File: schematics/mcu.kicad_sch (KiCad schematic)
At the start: 7 parts, among them SW1 SW_Push, U2 STM32F103C8Tx, Y1 ECS-2520MV-xxx-xx

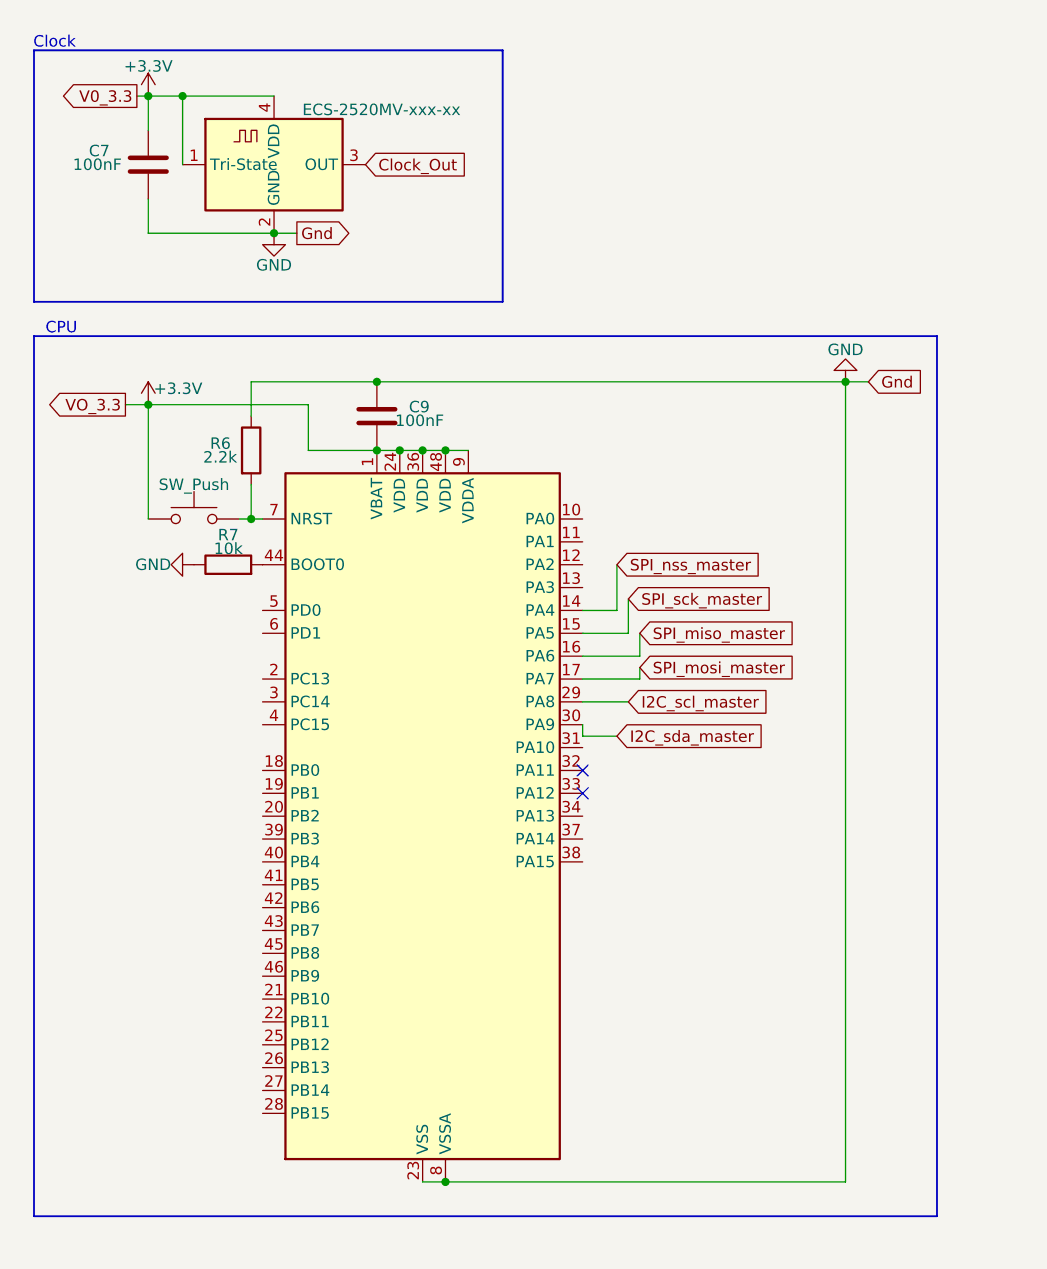
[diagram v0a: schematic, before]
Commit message: 2026-02-25 | Mi
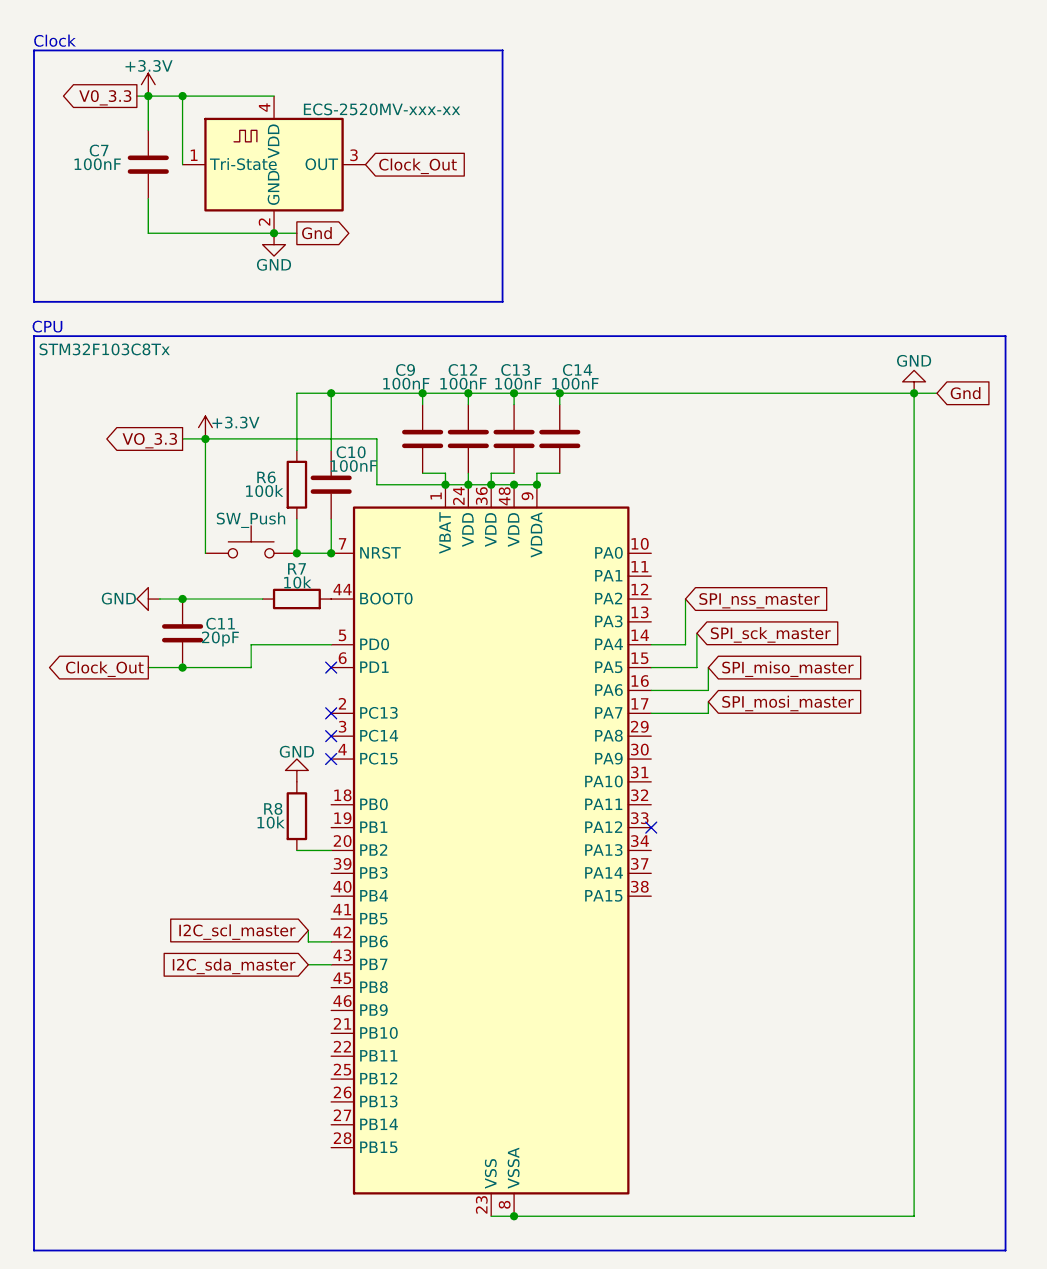
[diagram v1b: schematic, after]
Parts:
- added C10, C12, C13, C14: 100nF, Capacitor_SMD:C_0805_2012Metric, symbol Device:C
- added C11: 20pF, Capacitor_SMD:C_0805_2012Metric, symbol Device:C
- added R8: 10k, Resistor_SMD:R_0402_1005Metric, symbol Device:R
- R6: value 2.2k -> 100k
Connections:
- net +3.3V: now also C12.2, C13.2, C14.2
- net Clock_Out: now also U2.5 (PD0), C11.2
- net GND: now also C10.1, C11.1, C12.1, C13.1, C14.1, R8.1
- net I2C_scl_master: now also U2.42 (PB6); no longer U2.29 (PA8)
- net I2C_sda_master: now also U2.43 (PB7); no longer U2.30 (PA9)
- net at R6.2, SW1.2, U2.7 (NRST): now also C10.2
- net at U2.20 (PB2): now also R8.2
- no-connect marks 2 -> 5
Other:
- moved on the sheet: R6, R7

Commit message: 2026-02-26 | Do
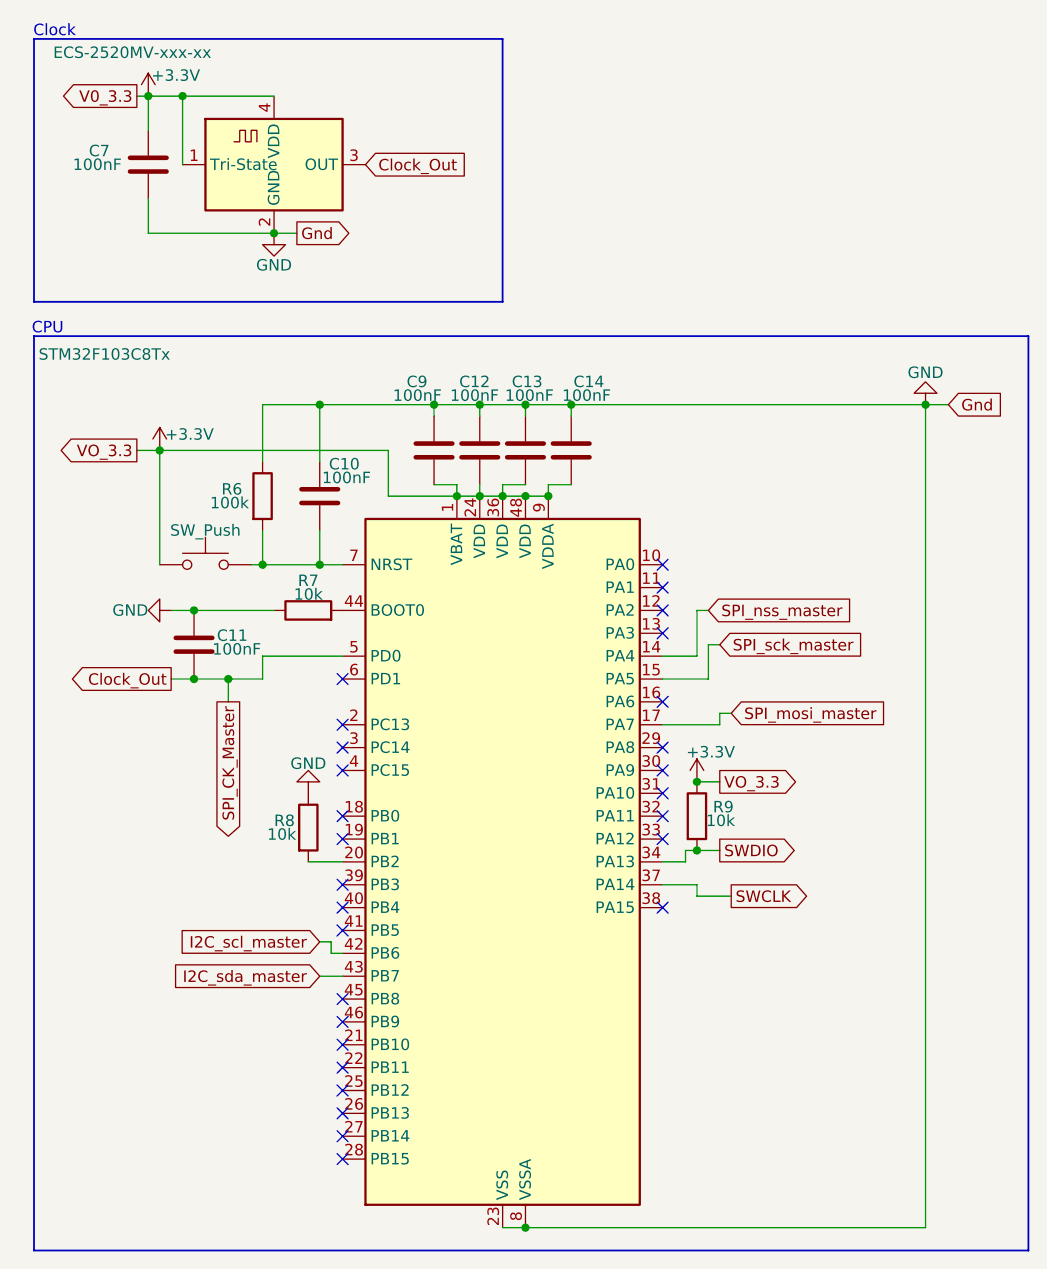
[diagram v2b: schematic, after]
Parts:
- added R9: 10k, Resistor_SMD:R_0402_1005Metric, symbol Device:R
- C11: value 20pF -> 100nF
- SW1: footprint Button_Switch_SMD:SW_Push_1P1T-SH_NO_CK_KMR2xxG -> Button_Switch_SMD:SW_Push_1P1T_NO_CK_KMR2
- Y1: footprint Oscillator:Oscillator_SMD_ECS_2520MV-xxx-xx-4Pin_2.5x2.0mm -> Oscillator:Oscillator_SMD_EuroQuartz_XO53-4Pin_5.0x3.2mm
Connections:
- net +3.3V: now also R9.1
- net SWDIO: now reaches U2.34 (PA13)
- net SWDIO: now also R9.2
- net SWCLK: now reaches U2.37 (PA14)
- net SPI_miso_master: no longer names the net of U2.16 (PA6)
- no-connect marks 5 -> 28
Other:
- moved on the sheet: C10, C11, C12, C13, C14, C9, R6, R7, R8
